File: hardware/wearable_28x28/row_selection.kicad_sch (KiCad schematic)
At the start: 101 parts, among them Q201 AO3403, Q202 AO3403, Q203 AO3403, Q204 AO3403, Q205 AO3403, Q206 AO3403, Q207 AO3403, Q208 AO3403, Q209 AO3403, Q210 AO3403, Q211 AO3403, Q212 AO3403, Q213 AO3403, Q214 AO3403, Q215 AO3403, Q216 AO3403, Q217 AO3403, Q218 AO3403, Q219 AO3403, Q220 AO3403, Q221 AO3403, Q222 AO3403, Q223 AO3403, Q224 AO3403, Q225 AO3403, Q226 AO3403, Q227 AO3403, Q228 AO3403, U201 SN74LVC8T245RHLR, U202 74HC154PW,118, U203 74HC154PW,118

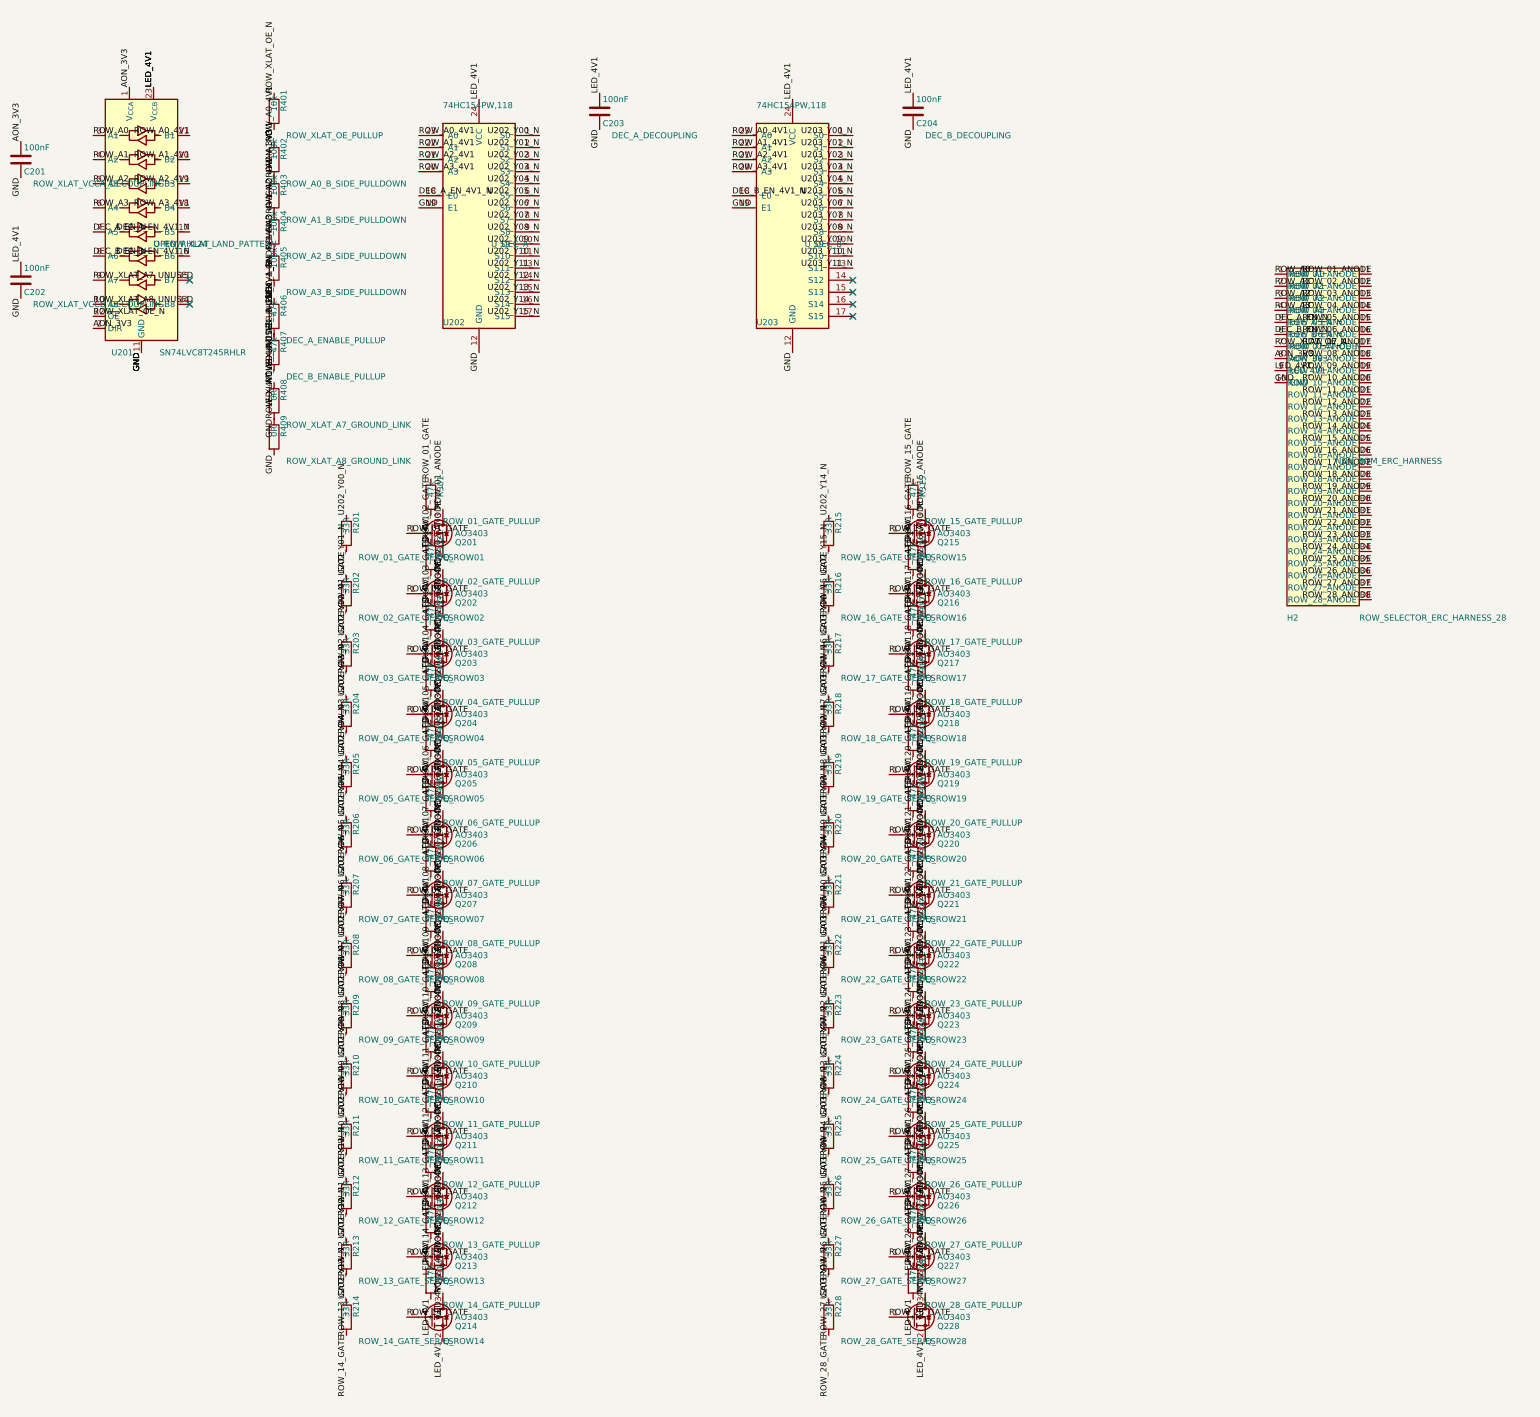
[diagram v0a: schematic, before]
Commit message: Separate row resistor label endpoints
Co-authored-by: illiapliukhin <illiapliukhin@users.noreply.github.com>
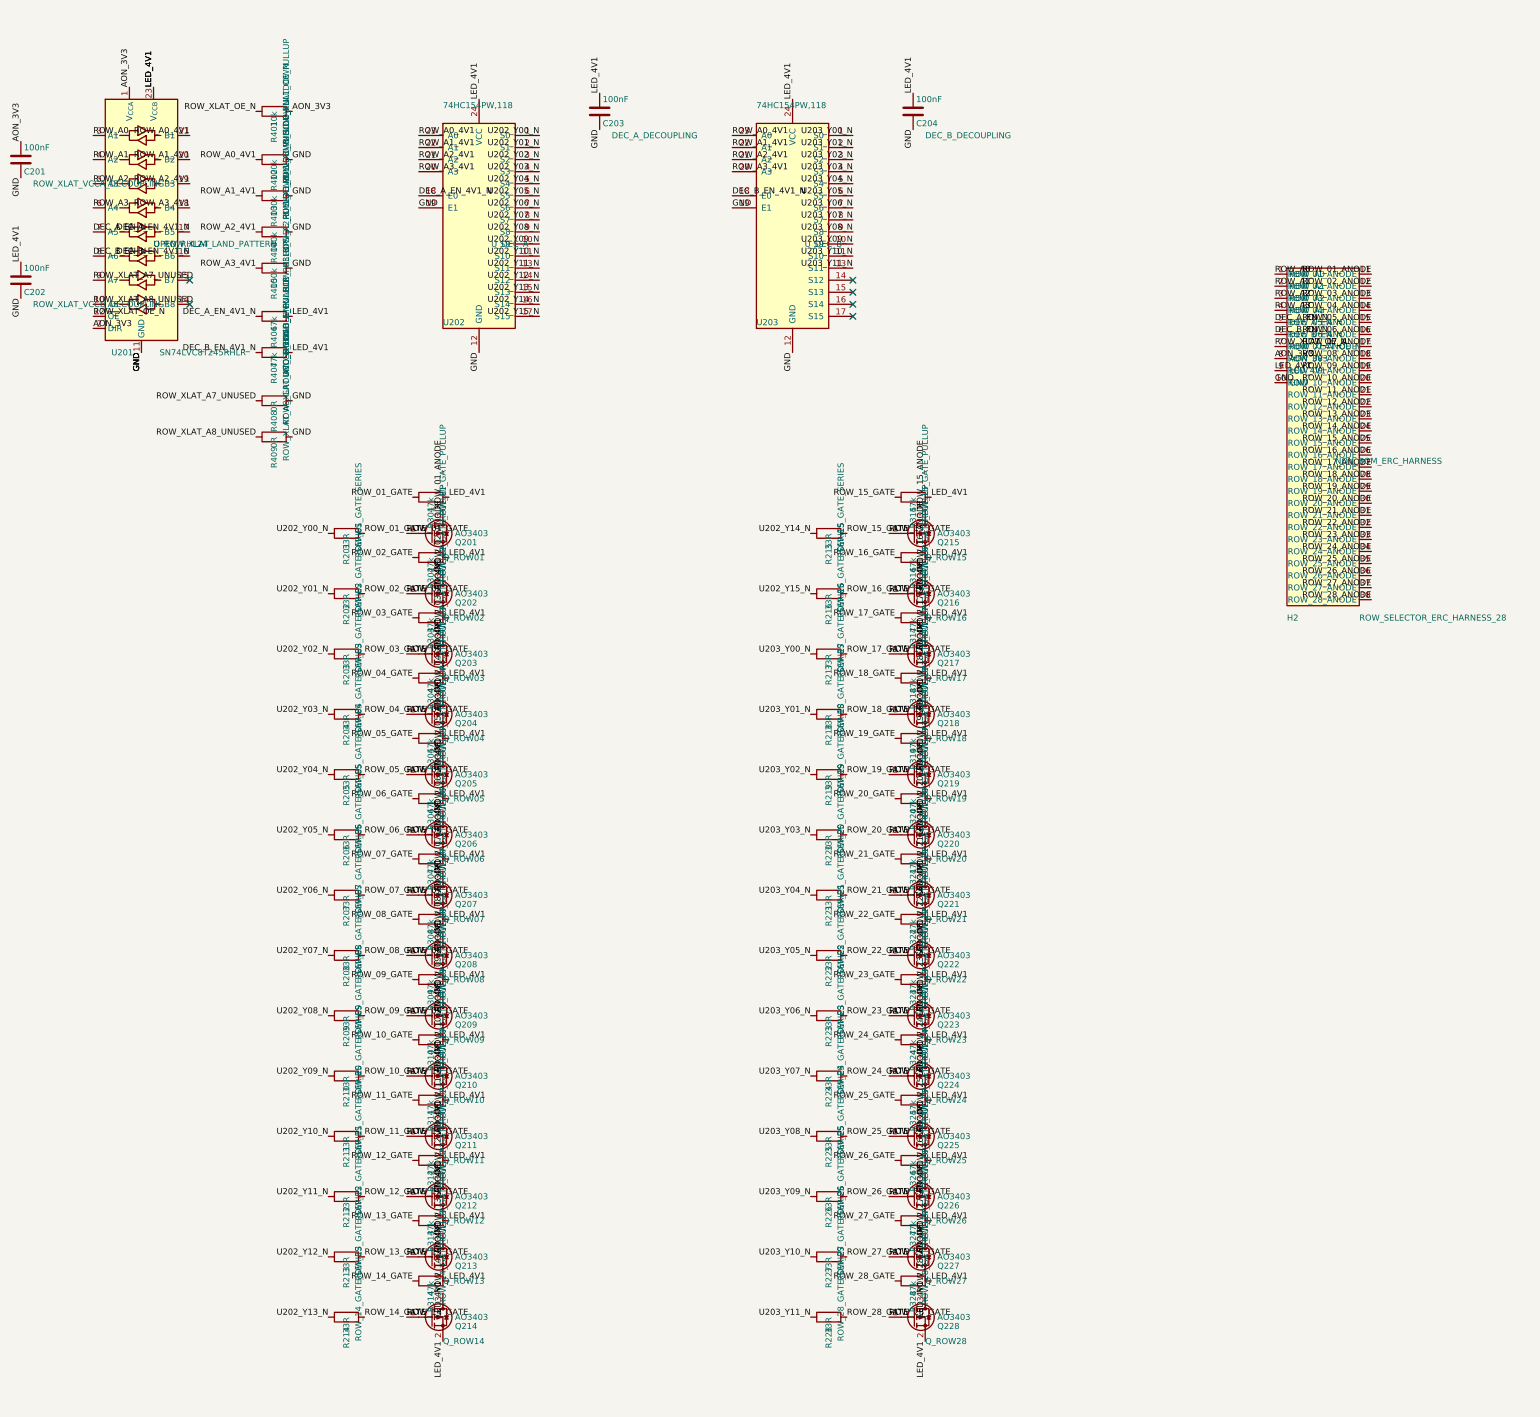
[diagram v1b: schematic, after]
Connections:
- net DEC_B_EN_4V1_N: no longer C202.1, C203.1, C204.1, H2.9 (LED_4V1), Q201.2 (S), Q202.2 (S), Q203.2 (S), Q204.2 (S), Q205.2 (S), Q206.2 (S), Q207.2 (S), Q208.2 (S), Q209.2 (S), Q210.2 (S), Q211.2 (S), Q212.2 (S), Q213.2 (S), Q214.2 (S), Q215.2 (S), Q216.2 (S), Q217.2 (S), Q218.2 (S), Q219.2 (S), Q220.2 (S), Q221.2 (S), Q222.2 (S), Q223.2 (S), Q224.2 (S), Q225.2 (S), Q226.2 (S), Q227.2 (S), Q228.2 (S), R301.2, R302.2, R303.2, R304.2, R305.2, R306.2, R307.2, R308.2, R309.2, R310.2, R311.2, R312.2, R313.2, R314.2, R315.2, R316.2, R317.2, R318.2, R319.2, R320.2, R321.2, R322.2, R323.2, R324.2, R325.2, R326.2, R327.2, R328.2, R406.2, R407.2, U201.23 (V_{CCB}), U201.24 (V_{CCB}), U202.24 (VCC), U203.24 (VCC)
- net GND: no longer R403.1, R404.1, R405.1, R409.1, U201.10 (A8), U201.18 (B4), U201.19 (B3), U201.20 (B2), U202.20 (A3), U202.21 (A2), U202.22 (A1), U203.20 (A3), U203.21 (A2), U203.22 (A1)
- new net LED_4V1: C202.1, C203.1, C204.1, H2.9 (LED_4V1), Q201.2 (S), Q202.2 (S), Q203.2 (S), Q204.2 (S), Q205.2 (S), Q206.2 (S), Q207.2 (S), Q208.2 (S), Q209.2 (S), Q210.2 (S), Q211.2 (S), Q212.2 (S), Q213.2 (S), Q214.2 (S), Q215.2 (S), Q216.2 (S), Q217.2 (S), Q218.2 (S), Q219.2 (S), Q220.2 (S), Q221.2 (S), Q222.2 (S), Q223.2 (S), Q224.2 (S), Q225.2 (S), Q226.2 (S), Q227.2 (S), Q228.2 (S), R301.2, R302.2, R303.2, R304.2, R305.2, R306.2, R307.2, R308.2, R309.2, R310.2, R311.2, R312.2, R313.2, R314.2, R315.2, R316.2, R317.2, R318.2, R319.2, R320.2, R321.2, R322.2, R323.2, R324.2, R325.2, R326.2, R327.2, R328.2, R406.2, R407.2, U201.23 (V_{CCB}), U201.24 (V_{CCB}), U202.24 (VCC), U203.24 (VCC)
- new net ROW_A1_4V1: R403.1, U201.20 (B2), U202.22 (A1), U203.22 (A1)
- new net ROW_A2_4V1: R404.1, U201.19 (B3), U202.21 (A2), U203.21 (A2)
- new net ROW_A3_4V1: R405.1, U201.18 (B4), U202.20 (A3), U203.20 (A3)
- new net ROW_XLAT_A8_UNUSED: R409.1, U201.10 (A8)
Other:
- moved on the sheet: R201, R202, R203, R204, R205, R206, R207, R208, R209, R210, R211, R212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
